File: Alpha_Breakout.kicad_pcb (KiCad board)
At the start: 4 copper layers, 66.7 x 74.4 mm, 161 parts, among them IC1 LM66200DRLR, J1 USB_C_Receptacle_USB2.0_14P, J10 Conn_01x03, J11 Conn_01x03, J12 Conn_01x03, J14 Conn_01x03, J15 Conn_01x03, J16 Conn_01x03, J18 Conn_01x02, J19 Conn_01x02, J20 Conn_01x02, J21 Conn_01x02, J22 Conn_01x02, J23 Conn_01x02, J24 Conn_01x04, J25 Conn_01x02, J26 Conn_01x02, J27 Conn_01x02, J28 Conn_01x02, J29 Conn_01x02, J3 Conn_01x03, J30 Conn_01x04, J31 Conn_01x02, J33 Conn_01x02, J34 Conn_01x02, J35 Conn_02x06_Odd_Even, J36 Conn_01x02, J4 Conn_01x03, J5 Conn_01x03, J7 Conn_01x03, J8 Conn_01x03, J9 Conn_01x03, Q1 CSD13381F4, Q2 CSD13381F4, Q3 CSD13381F4, Q4 CSD13381F4, Q5 SSM3J328R, Q6 L2N7002SLLT1G, SW1 SW_Push, SW2 SW_Push, U1 STM32F103C8Tx, U10 LP2985-3.3, U11 SP3485EN, U12 ADS1231ID, U13 TCA9517ADGK, U2 CH340N, U3 ADS7828, U4 ADS7828, U5 MAX31856, U6 MAX31856, U7 MAX31856, U8 MAX31856, U9 AP63203WU

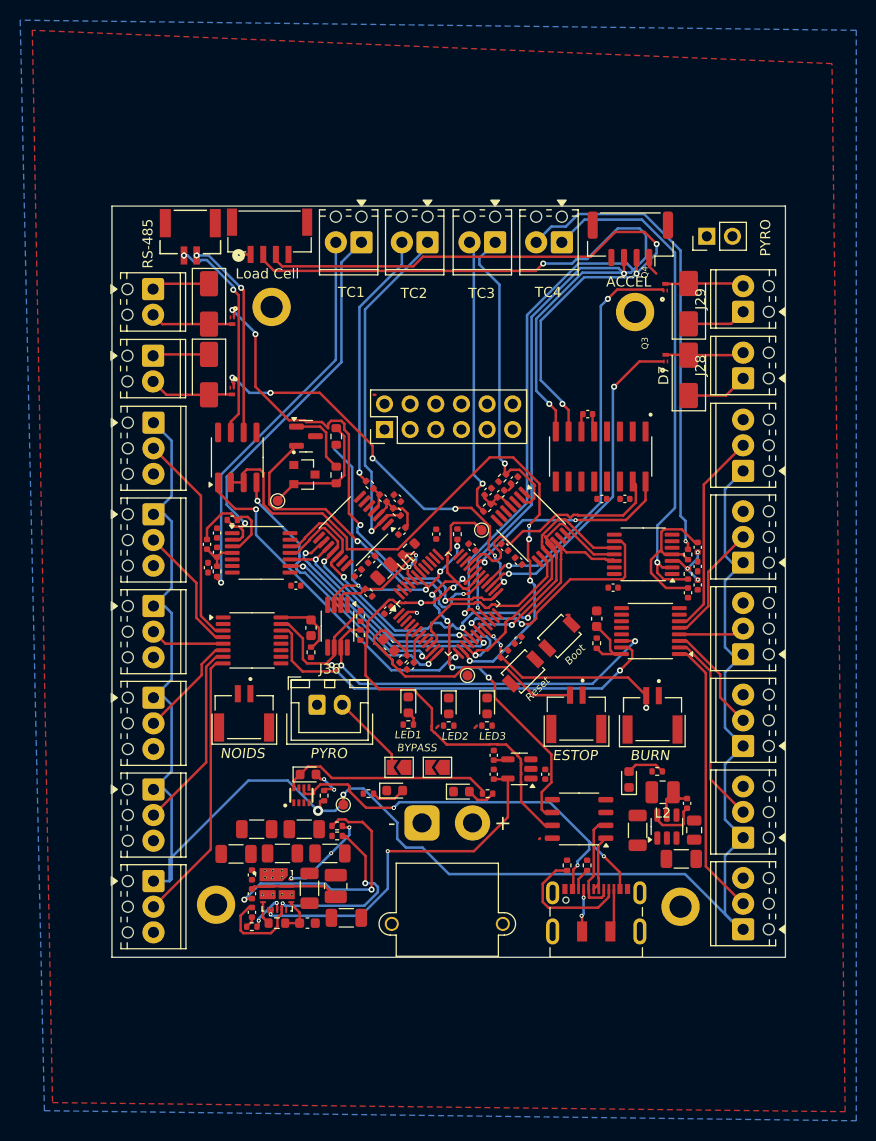
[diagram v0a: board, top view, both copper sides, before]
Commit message: parts⚙️
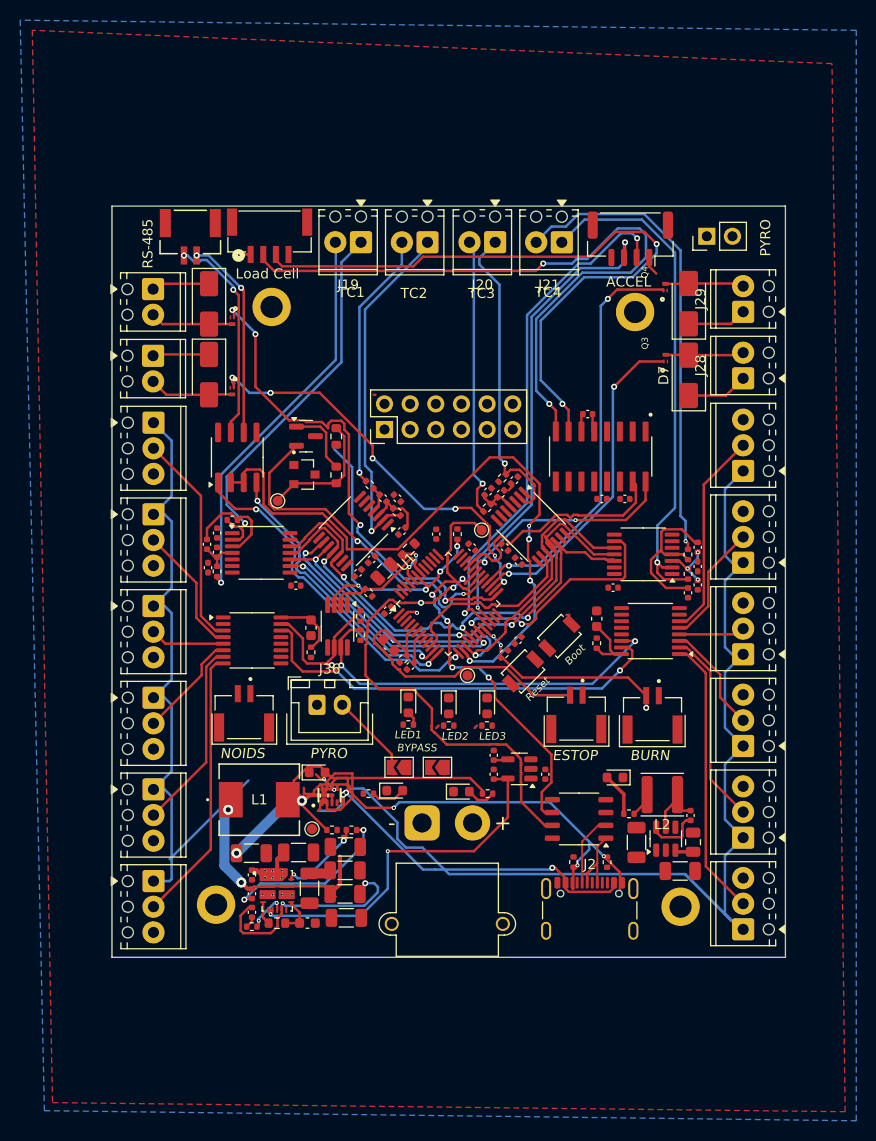
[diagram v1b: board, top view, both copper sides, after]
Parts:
- removed J1: USB_C_Receptacle_USB2.0_14P, Connector_USB:USB_C_Receptacle_JAE_DX07S016JA1R1500
- added J2: USB_C_Receptacle_USB2.0_16P, Connector_USB:USB_C_Receptacle_GCT_USB4105-xx-A_16P_TopMnt_Horizontal, F.Cu at (162.4, 133.0)
- D1, D2: value LED -> White
- D10: value Yellow -> White
- D4: value GREEN -> White
- L1: footprint Inductor_SMD:L_1008_2520Metric -> CYA0630-1.5UH:IND_CYA0630_SHH
- L2: footprint Inductor_SMD:L_1008_2520Metric -> Inductor_SMD:L_Changjiang_FNR4030S
- R20, R21: value 200 -> 100
- moved L1 11.4 mm to (129.7, 121.1), turned to 0 degrees
- moved C40 10.8 mm to (138.2, 125.8), turned to 0 degrees
- moved C35 9.65 mm to (138.2, 128.1)
- moved C34 7.38 mm to (138.2, 130.4)
- moved C39 5.74 mm to (128.9, 126.4)
- moved R18 5.05 mm to (166.3, 122.5), turned to 180 degrees
- moved R4 3.98 mm to (164.1, 127.3)
- moved TP4 3.92 mm to (134.9, 124.0)
- moved C37 3.11 mm to (133.6, 126.3)
- moved IC1 2.79 mm to (136.6, 120.7)
- moved R15 1.48 mm to (138.8, 124.1), turned to 180 degrees
- moved D1 1.40 mm to (164.9, 118.9), turned to 180 degrees
- moved R5 1.39 mm to (160.8, 127.3)
- moved C38 1.25 mm to (172.4, 122.7)
- moved C41 1.21 mm to (167.0, 125.3)
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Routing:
- net Net-(J18-Pin_1): track 35.0 -> 78.9 mm, vias 1 -> 5
- net SDA_5V: track 48.5 -> 13.6 mm, vias 2 -> 0
- net /ADS1231/LC_DRDY/DOUT: track 22.4 -> 57.2 mm, vias 2 -> 4
- net /Solenoids/S4: track 41.1 -> 8.94 mm
- net /Breakout/PB5: track 0.00 -> 32.1 mm
- net /Hardware_Safe/K1: track 31.0 -> 2.95 mm
- net BATT_V+: track 0.00 -> 20.1 mm, vias 0 -> 2
- net PYRO_PWR: track 8.23 -> 28.0 mm
- net Net-(J2-CC2): track 12.8 -> 0.00 mm
- net Net-(C31-Pad2): track 8.88 -> 19.4 mm, vias 0 -> 2
- net (no net): track 8.72 -> 0.07 mm, vias 2 -> 0
- net unconnected-(J2-SBU2-PadB8): track 0.00 -> 8.23 mm
- net USB_V+: track 43.9 -> 35.8 mm, vias 4 -> 2
- net Net-(C31-Pad1): track 24.8 -> 17.0 mm
- net +BATT: track 0.00 -> 6.99 mm
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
